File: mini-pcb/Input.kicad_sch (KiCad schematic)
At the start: 18 parts, among them U2 OPA1664D, U3 OPA1655DBV

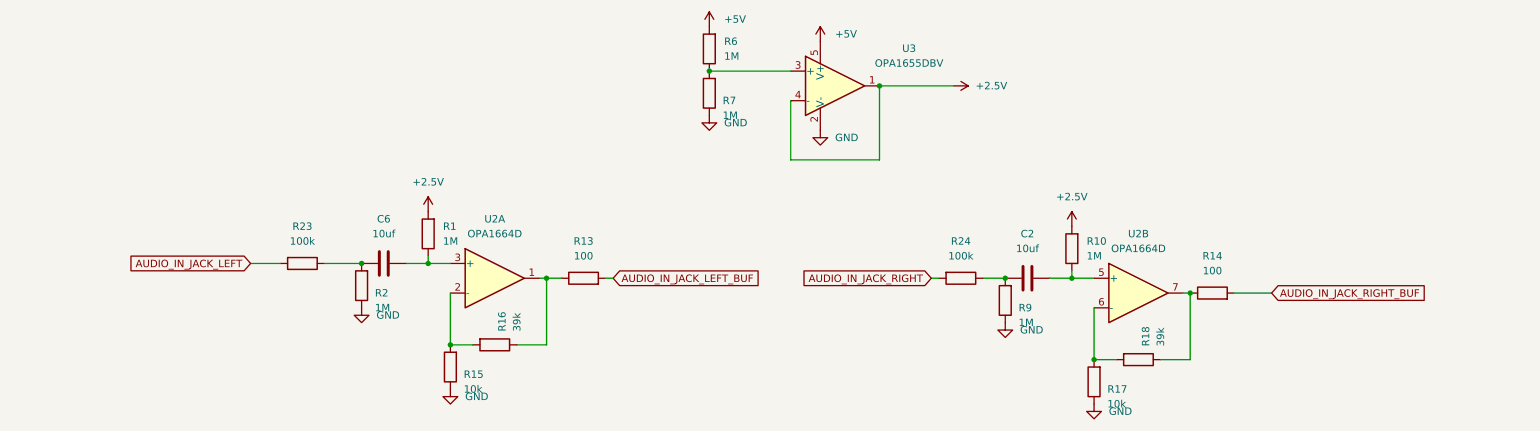
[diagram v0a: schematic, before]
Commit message: ordered pcb
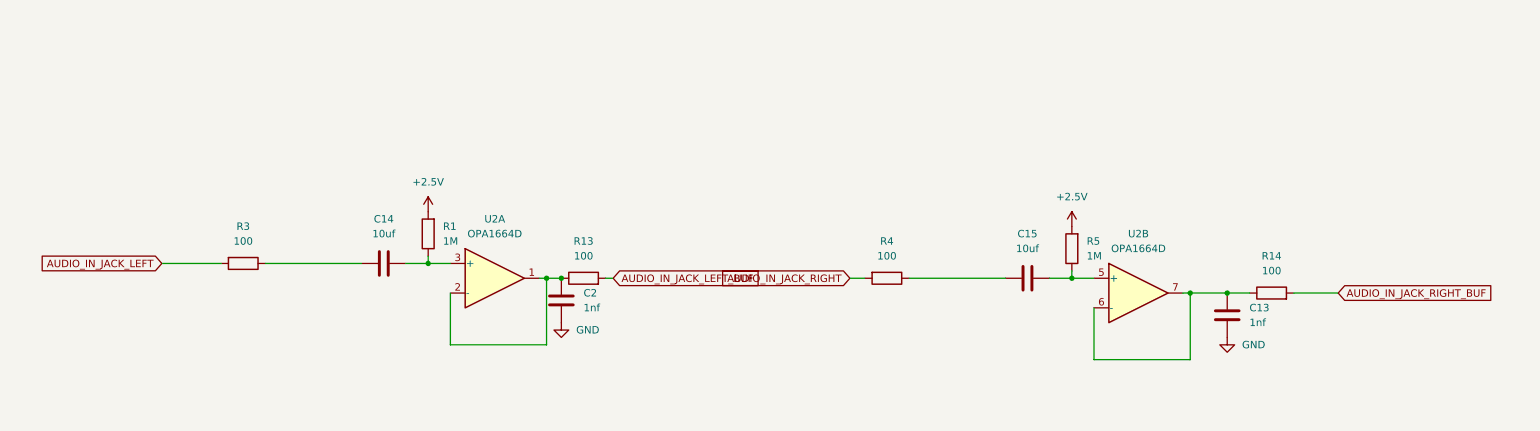
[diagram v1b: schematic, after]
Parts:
- removed C6: 10uf, Capacitor_SMD:C_0805_2012Metric, symbol Device:C
- removed R10, R2, R6, R7, R9: 1M, Resistor_SMD:R_0603_1608Metric, symbol Device:R
- removed R15, R17: 10k, Resistor_SMD:R_0603_1608Metric, symbol Device:R
- removed R16, R18: 39k, Resistor_SMD:R_0603_1608Metric, symbol Device:R
- removed R23, R24: 100k, Resistor_SMD:R_0603_1608Metric, symbol Device:R
- removed U3: OPA1655DBV, Package_TO_SOT_SMD:SOT-23-5, symbol Amplifier_Operational:OPA1655DBV
- added C13: 1nf, Capacitor_SMD:C_0805_2012Metric, symbol Device:C
- added C14, C15: 10uf, Capacitor_SMD:C_0805_2012Metric, symbol Device:C
- added R3, R4: 100, Resistor_SMD:R_0603_1608Metric, symbol Device:R
- added R5: 1M, Resistor_SMD:R_0603_1608Metric, symbol Device:R
- C2: value 10uf -> 1nf; MPN (none) -> C46653
- R1: MPN (none) -> C22935
- R13, R14: MPN (none) -> C22775
- U2: MPN (none) -> C69414
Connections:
- net +2.5V: now also R5.2
- net AUDIO_IN_JACK_LEFT: now also R3.2
- net AUDIO_IN_JACK_RIGHT: now also R4.2
- net GND: now also C2.1, C13.1
- net at R1.1, U2.3 (+): now also C14.2
- net at U2.2 (-): now also C2.2, R13.1, U2.1
- net at R14.1, U2.7: now also U2.6 (-), C13.2
- net at U2.5 (+): now also C15.2, R5.1; no longer C2.2
- new net: C15.1, R4.1
- new net: C14.1, R3.1

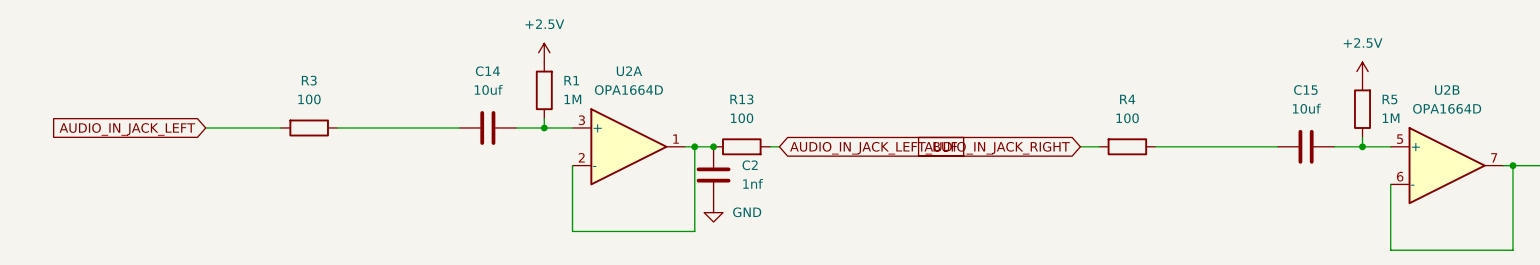
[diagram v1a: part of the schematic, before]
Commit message: made mini-pcb report
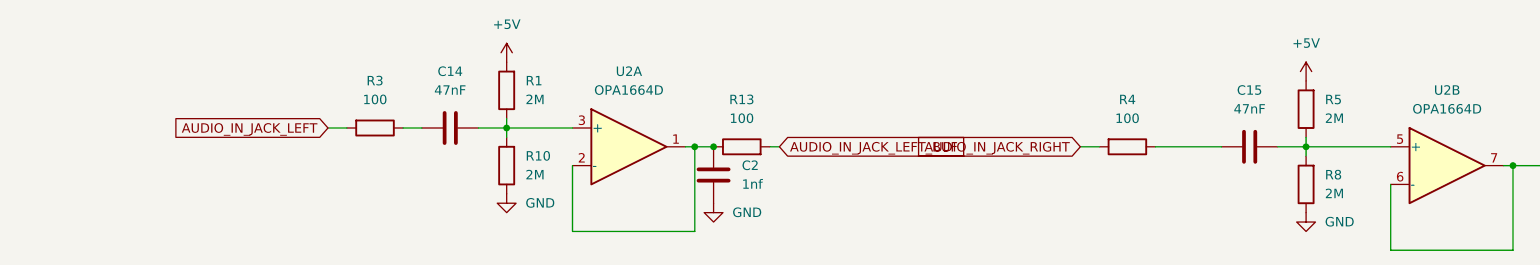
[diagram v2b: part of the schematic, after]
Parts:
- added R10, R8: 2M, Resistor_SMD:R_0603_1608Metric, symbol Device:R
- C14, C15: value 10uf -> 47nF; MPN C440198 -> C2182212
- R1, R5: value 1M -> 2M; MPN C22935 -> C22976
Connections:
- net GND: now also R10.1, R8.1
- net at C14.2, R1.1, U2.3 (+): now also R10.2
- net at C15.2, R5.1, U2.5 (+): now also R8.2
- net +2.5V renamed +5V
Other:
- moved on the sheet: C14, C15, R1, R3, R5
